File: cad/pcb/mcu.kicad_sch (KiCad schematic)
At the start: 34 parts, among them X4 SWD-Conn, X5 UART_Conn, Y1 32MHz, Y2 32.768k

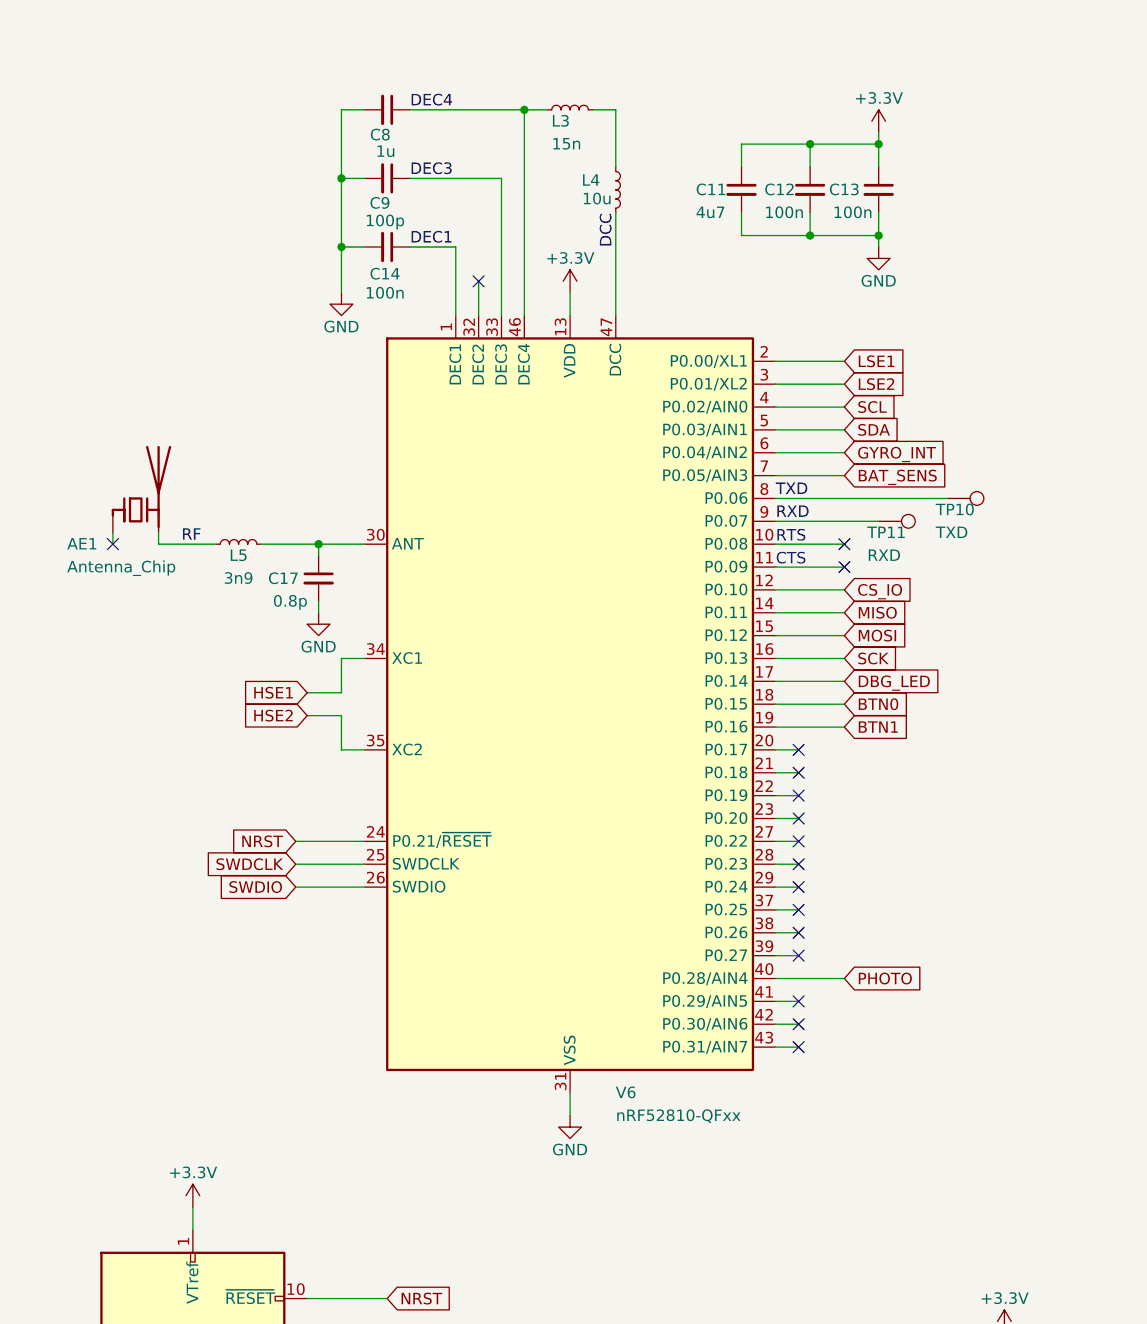
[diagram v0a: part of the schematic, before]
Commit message: add pcb layout
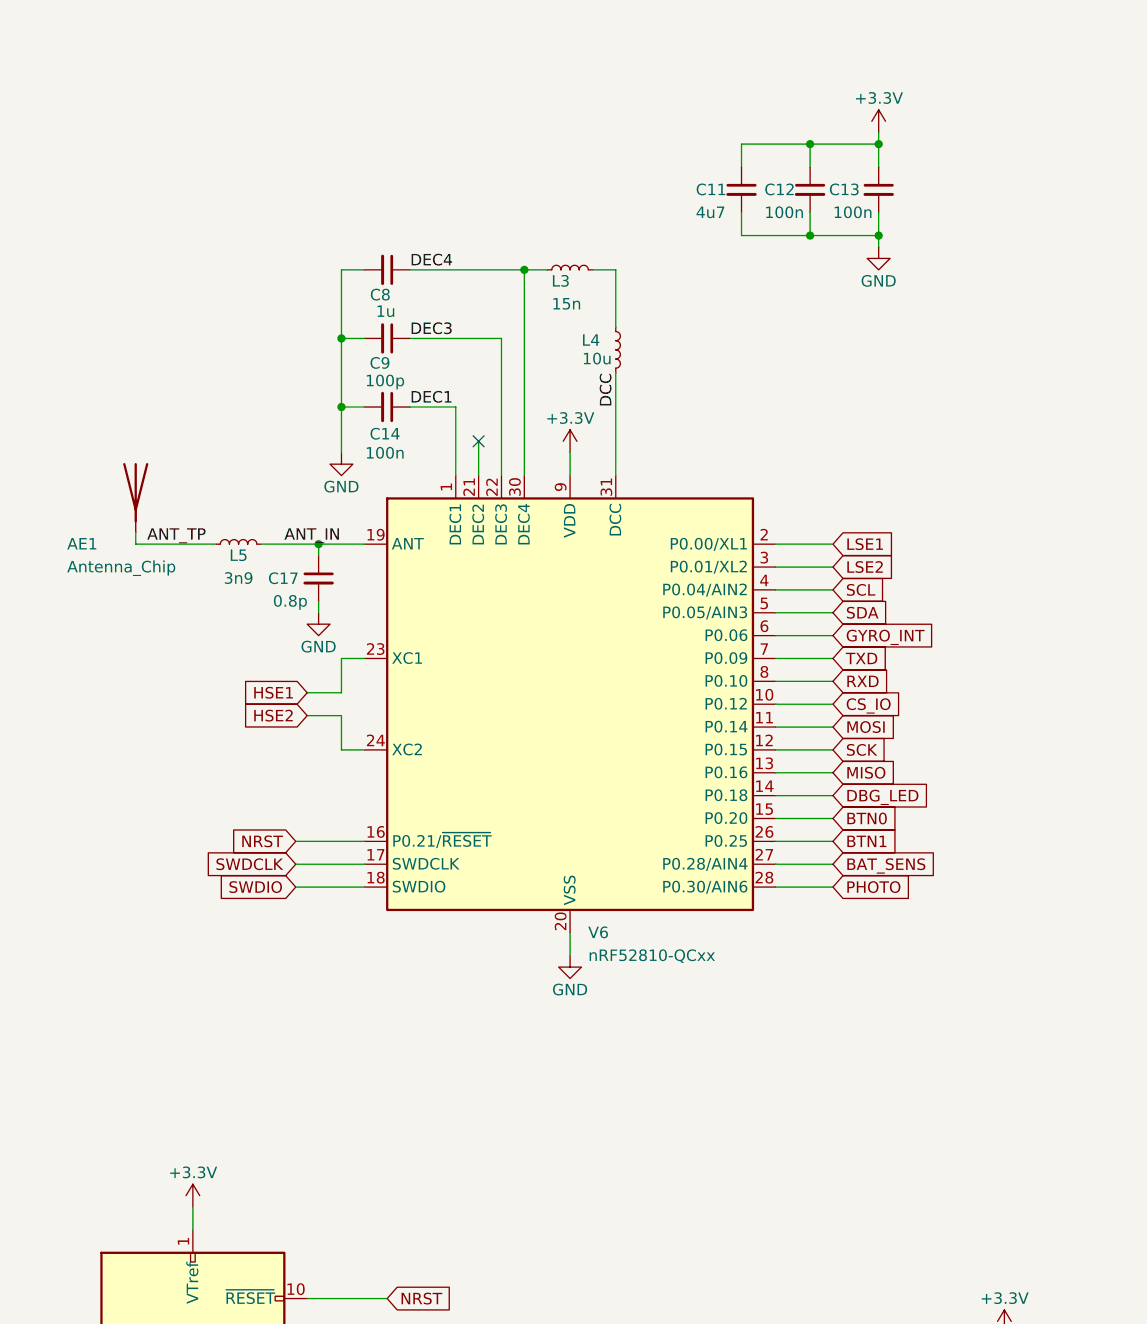
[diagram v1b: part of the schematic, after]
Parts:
- removed AE1: Antenna_Chip, myLib:Ignion_NN01-102_BT_WIFI, symbol Device:Antenna_Chip
- removed TP10: TXD, TestPoint:TestPoint_Pad_D1.0mm, symbol Connector:TestPoint
- removed TP11: RXD, TestPoint:TestPoint_Pad_D1.0mm, symbol Connector:TestPoint
- removed V6: nRF52810-QFxx, Package_DFN_QFN:QFN-48-1EP_6x6mm_P0.4mm_EP4.6x4.6mm, symbol MCU_Nordic:nRF52810-QFxx
- added AE1: Antenna_Chip, myLib:Ignion_NN01-102_BT_WIFI, symbol Device:Antenna
- added V6: nRF52810-QCxx, Package_DFN_QFN:QFN-32-1EP_5x5mm_P0.5mm_EP3.6x3.6mm, symbol MCU_Nordic:nRF52810-QCxx
- S1: footprint Button_Switch_SMD:SW_SPST_CK_RS282G05A3 -> myLib:Tactile_E-Switch_TL3780AF240QG
- S2, S3: footprint Button_Switch_SMD:SW_SPST_CK_RS282G05A3 -> myLib:Tactile_Panasonic_EVQ-P7J01P
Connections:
- net +3.3V: now also V6.25 (VDD), V6.32 (VDD), V6.9 (VDD)
- net BAT_SENS: now also V6.27 (P0.28/AIN4)
- net BTN0: now also V6.15 (P0.20)
- net BTN1: now also V6.26 (P0.25)
- net CS_IO: now also V6.10 (P0.12)
- net DBG_LED: now also V6.14 (P0.18)
- net DCC: now also V6.31 (DCC)
- net DEC1: now also V6.1 (DEC1)
- net DEC3: now also V6.22 (DEC3)
- net DEC4: now also V6.30 (DEC4)
- net GND: now also V6.20 (VSS), V6.29 (VSS), V6.33 (VSS)
- net GYRO_INT: now also V6.6 (P0.06)
- net HSE1: now also V6.23 (XC1)
- net HSE2: now also V6.24 (XC2)
- net LSE1: now also V6.2 (P0.00/XL1)
- net LSE2: now also V6.3 (P0.01/XL2)
- net MISO: now also V6.13 (P0.16)
- net MOSI: now also V6.11 (P0.14)
- net NRST: now also V6.16 (P0.21/~{RESET})
- net PHOTO: now also V6.28 (P0.30/AIN6)
- net RXD: now also V6.8 (P0.10)
- net SCK: now also V6.12 (P0.15)
- net SCL: now also V6.4 (P0.04/AIN2)
- net SDA: now also V6.5 (P0.05/AIN3)
- net SWDCLK: now also V6.17 (SWDCLK)
- net SWDIO: now also V6.18 (SWDIO)
- net TXD: now also V6.7 (P0.09)
- net ANT_IN: now reaches C17.1, L5.2
- net ANT_IN: now also V6.19 (ANT)
- net RF renamed ANT_TP
- net ANT_TP: now also AE1.1 (A)
- no-connect marks 20 -> 4
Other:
- note removed: "CTS"
- note removed: "RTS"
- moved on the sheet: C14, C8, C9, L3, L4
